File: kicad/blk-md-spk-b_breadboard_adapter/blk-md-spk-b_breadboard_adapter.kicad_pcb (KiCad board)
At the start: 2 copper layers, 26.4 x 39.1 mm, 4 parts, among them J1 SCJ-0354-5PU, P1 CONNECTOR, P2 CONNECTOR, U1 BLK-MD-SPK-B

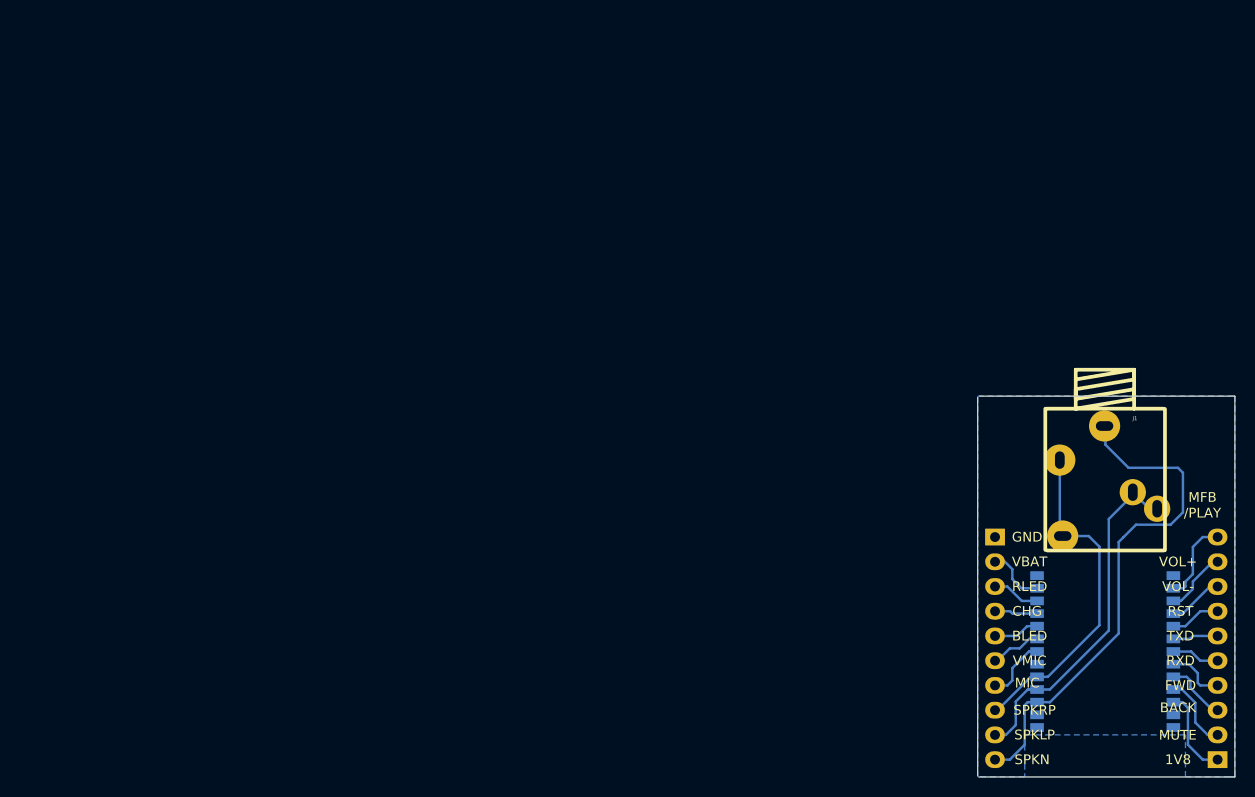
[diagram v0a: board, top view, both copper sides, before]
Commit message: udpated to version 2.1
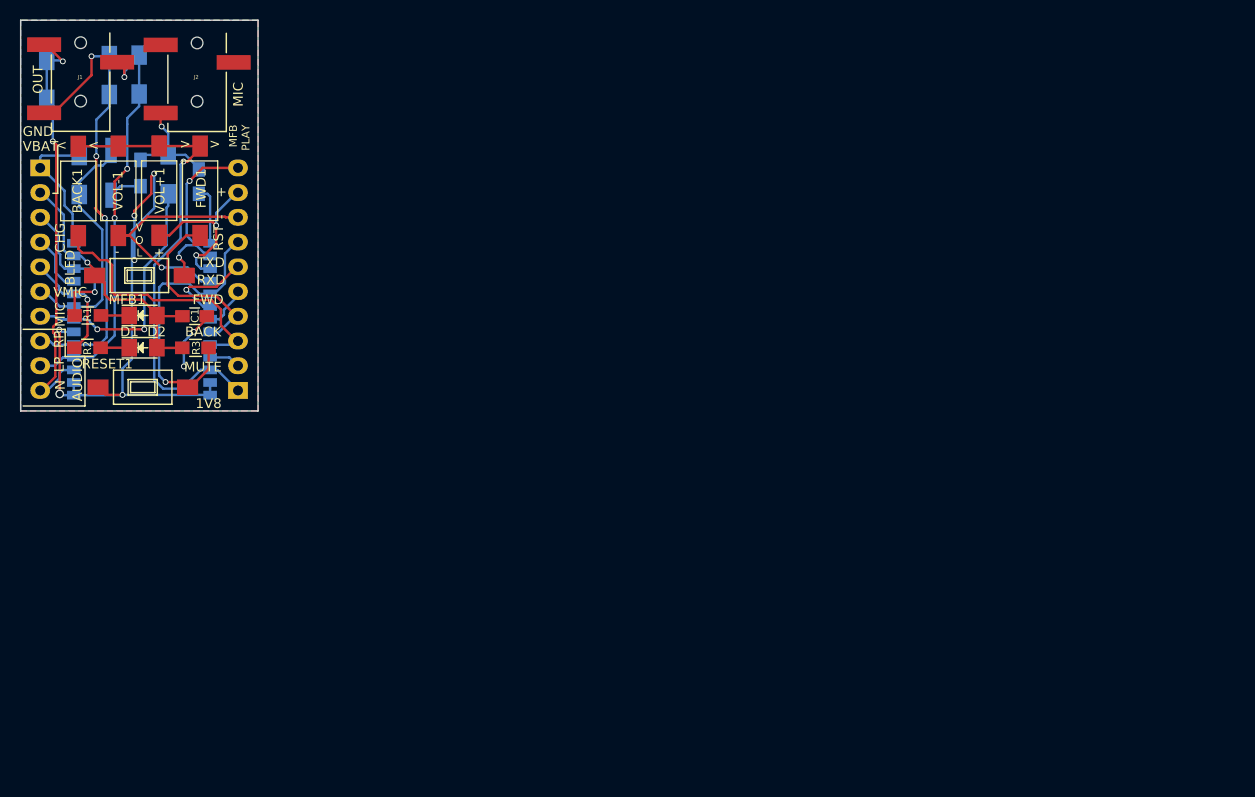
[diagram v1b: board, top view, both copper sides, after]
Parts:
- added BACK1: SW_PUSH, Buttons_Switches_SMD:SW_SPST_FSMSM, F.Cu at (115.6, 108.2)
- added C1: 100n, Capacitors_SMD:C_0805_HandSoldering, F.Cu at (127.6, 121.1)
- added C2: 4u7, Capacitors_SMD:C_1206_HandSoldering, B.Cu at (115.7, 106.6)
- added C3: 1u, Capacitors_SMD:C_1206_HandSoldering, B.Cu at (124.9, 106.5)
- added C4: 10, Capacitors_SMD:C_0805_HandSoldering, B.Cu at (128.0, 107.3)
- added C5: 1u, Capacitors_SMD:C_1206_HandSoldering, B.Cu at (112.4, 96.8)
- added C6: 1u, Capacitors_SMD:C_1206_HandSoldering, B.Cu at (118.8, 96.3)
- added C7: 1u, Capacitors_SMD:C_1206_HandSoldering, B.Cu at (121.9, 96.3)
- added D1: LED, LEDs:LED-1206, F.Cu at (122.3, 121.0)
- added D2: LED, LEDs:LED-1206, F.Cu at (122.3, 124.3)
- added FWD1: SW_PUSH, Buttons_Switches_SMD:SW_SPST_FSMSM, F.Cu at (128.2, 108.2)
- added J2: Jack_3.5mm_3pin, jacks:3.5mm_stereo_jack_PJ320B, F.Cu at (127.9, 93.0)
- added L1: 15n, Choke_SMD.pretty:Choke_SMD_1206_Handsoldering, B.Cu at (119.0, 106.4)
- added MFB1: SW_PUSH, Buttons_Switches_SMD:SW_SPST_FSMSM, F.Cu at (121.9, 116.9)
- added R1: 470, Resistors_SMD:R_0805_HandSoldering, F.Cu at (116.6, 121.0)
- added R2: 470, Resistors_SMD:R_0805_HandSoldering, F.Cu at (116.6, 124.3)
- added R3: 10k, Resistors_SMD:R_0805_HandSoldering, F.Cu at (127.7, 124.3)
- added R4: 2k7, Resistors_SMD:R_0805_HandSoldering, B.Cu at (122.0, 106.4)
- added RESET1: SW_PUSH, Buttons_Switches_SMD:SW_SPST_FSMSM, F.Cu at (122.3, 128.4)
- added VOL+1: SW_PUSH, Buttons_Switches_SMD:SW_SPST_FSMSM, F.Cu at (124.0, 108.2)
- added VOL-1: SW_PUSH, Buttons_Switches_SMD:SW_SPST_FSMSM, F.Cu at (119.8, 108.2)
- J1: value SCJ-0354-5PU -> Jack_3.5mm_3pin; footprint jacks:SCJ-0354-5PU -> jacks:3.5mm_stereo_jack_PJ320B
- U1: footprint my_modules:BLK-MD-SPK-B -> my_modules:BLK-MD-SPK-B_no_up_silk
- moved J1 111.7 mm to (115.9, 93.0)
- moved P2 109.8 mm to (111.7, 105.8), turned to 180 degrees
- moved U1 104.7 mm to (113.9, 135.5)
- moved P1 104.0 mm to (132.1, 128.7), turned to 0 degrees
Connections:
- net Net-(J1-Pad1) renamed /SPKN
- net Net-(P1-Pad1) renamed /1V8
- net Net-(P1-Pad10) renamed /MFB
- net Net-(P1-Pad2) renamed /MUTE
- net Net-(P1-Pad3) renamed /BACK
- net Net-(P1-Pad4) renamed /FWD
- net Net-(P1-Pad5) renamed /RXD
- net Net-(P1-Pad6) renamed /TXD
- net Net-(P1-Pad7) renamed /RST
- net Net-(P1-Pad8) renamed /VOL-
- net Net-(P1-Pad9) renamed /VOL+
- net Net-(P2-Pad2) renamed /VBAT
- net Net-(P2-Pad3) renamed /RLED
- net Net-(P2-Pad4) renamed /CHG
- net Net-(P2-Pad5) renamed /BLED
- net Net-(P2-Pad6) renamed /VMIC
- net Net-(P2-Pad7) renamed /MIC
- J1 pad 2: Net-(J1-Pad2) -> /SPKRP
- J1 pad 3: Net-(J1-Pad2) -> /SPKLP
- P2 pad 8: Net-(J1-Pad4) -> /SPKRP
- P2 pad 9: Net-(J1-Pad2) -> /SPKLP
- U1 pad 14: (no net) -> GND
- U1 pad 4: Net-(J1-Pad2) -> /SPKLP
- U1 pad 5: Net-(J1-Pad4) -> /SPKRP
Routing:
- net GND: track 0.00 -> 90.2 mm, vias 0 -> 8
- net /SPKRP: track 0.00 -> 49.6 mm, vias 0 -> 3
- net /SPKLP: track 0.00 -> 44.0 mm, vias 0 -> 3
- net /1V8: track 8.71 -> 49.5 mm, vias 0 -> 1
- net Net-(J1-Pad2): track 37.3 -> 0.00 mm
- net Net-(J1-Pad4): track 34.7 -> 0.00 mm
- net /RST: track 4.67 -> 31.8 mm, vias 0 -> 1
- net /VBAT: track 6.62 -> 29.8 mm, vias 0 -> 1
- net /BACK: track 5.90 -> 28.1 mm
- net /MIC: track 6.50 -> 26.9 mm, vias 0 -> 2
- net /VMIC: track 5.25 -> 25.2 mm
- net /VOL-: track 5.18 -> 24.5 mm, vias 0 -> 1
- net /FWD: track 5.53 -> 19.6 mm
- net /VOL+: track 6.14 -> 19.6 mm, vias 0 -> 2
- net /RLED: track 4.93 -> 16.6 mm, vias 0 -> 1
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- added copper zone on F.Cu, net GND
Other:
- board size 26.4 x 39.1 mm -> 24.4 x 40.1 mm
- net class Default: clearance 0.254 -> 0.2; trace_width 0.254 -> 0.25; via_dia 0.889 -> 0.6; via_drill 0.635 -> 0.4
- rule pad_to_mask_clearance: 0 -> 0.2
- rule trace_clearance: 0.254 -> 0.2
- rule trace_min: 0.254 -> 0.2
- rule via_min_drill: 0.508 -> 0.3
- rule via_min_size: 0.889 -> 0.4
- board text added: "+"
- board text added: "-"
- board text added: "<"
- board text added: ">"
- board text added: "AUDIO"
- board text added: "LP"
- board text added: "MFB PLAY"
- board text added: "N"
- board text added: "OUT"
- board text added: "RP"
- board text added: "V O L"
- board text removed: "MFB /PLAY"
- board text removed: "RLED"
- board text removed: "SPKLP"
- board text removed: "SPKN"
- board text removed: "SPKRP"
- board text removed: "VOL+"
- board text removed: "VOL-"
